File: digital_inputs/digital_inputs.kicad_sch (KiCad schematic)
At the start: 147 parts, among them J1 6437288-2, J10 Conn_01x01, J11 Conn_01x01, J12 Conn_01x01, J13 Conn_01x01, J14 Conn_01x01, J15 Conn_01x01, J16 Conn_01x01, J17 Conn_01x01, J18 Conn_02x05_Odd_Even, J19 6437288-3, J2 Conn_02x07_Odd_Even, J20 Conn_02x24_Odd_Even, J21 Conn_02x08_Odd_Even, J22 Conn_02x15_Odd_Even, J23 Conn_02x10_Odd_Even, J24 Conn_02x17_Odd_Even, J25 Conn_02x10_Odd_Even, J26 Conn_02x06_Odd_Even, J27 Conn_02x16_Odd_Even, J28 Conn_02x04_Odd_Even, J3 Conn_01x08, J4 Conn_01x01, J5 Conn_01x02, J6 Conn_01x04, J7 Conn_01x04, J8 Conn_01x04, J9 Conn_01x04, Q1 AO3400A, Q2 AO3400A, Q3 AO3400A, Q4 AO3400A, Q5 AO3400A, Q6 AO3400A, Q7 AO3400A, Q8 AO3400A, U1 OPA4192IPW, U10 ULN2003A, U12 TJA1051T-3, U2 CD4067BM96, U3 CD4067BM96, U4 CD4067BM96, U5 CD4067BM96, U6 CD4067BM96, U7 CD4067BM96, U8 TC4427, U9 TC4427

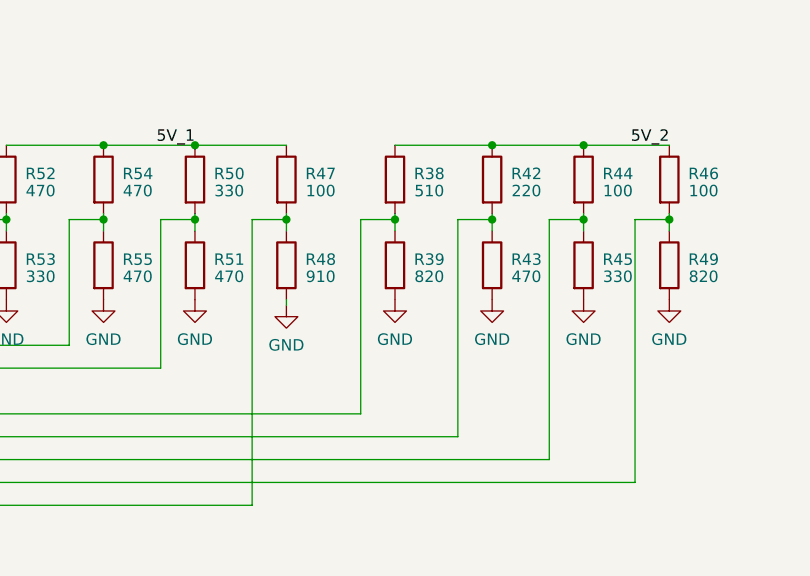
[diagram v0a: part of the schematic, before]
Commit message: check
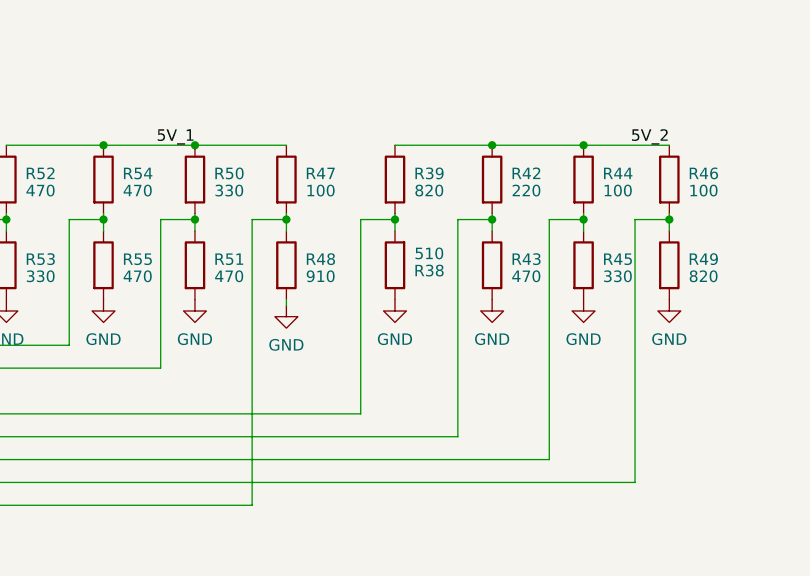
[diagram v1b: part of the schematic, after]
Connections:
- net 5V_2: now also R39.1; no longer R38.1
- net GND: now also R38.1; no longer R39.2
- net REF12: now also R39.2; no longer R39.1
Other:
- moved on the sheet: R38, R39
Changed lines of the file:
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@@
     (stroke (width 0) (type default))
   )
-  (wire (pts (xy 127 356.87) (xy 127 335.28))
+  (wire (pts (xy 127 335.28) (xy 127 356.87))
     (stroke (width 0) (type default))
   )
@@
     )
   )
-  (symbol (lib_id "Device:R") (at 130.81 340.36 0) (unit 1)
-    (in_bom yes) (on_board yes) (dnp no)
-    (property "Reference" "R39" (at 134.62 339.725 0)
-      (effects (font (size 1.27 1.27)))
-    )
-    (property "Value" "820" (at 134.62 341.63 0)
-      (effects (font (size 1.27 1.27)))
-    )
-    (property "Footprint" "Resistor_SMD:R_0603_1608Metric" (at 129.032 340.36 90)
-      (effects (font (size 1.27 1.27)) hide)
-    )
-    (property "Datasheet" "~" (at 130.81 340.36 0)
-      (effects (font (size 1.27 1.27)) hide)
-    )
-    (property "LCSC" "C23253" (at 130.81 340.36 0)
+  (symbol (lib_id "Device:R") (at 130.81 330.835 0) (unit 1)
+    (in_bom yes) (on_board yes) (dnp no)
+    (property "Reference" "R39" (at 134.62 330.2 0)
+      (effects (font (size 1.27 1.27)))
+    )
+    (property "Value" "820" (at 134.62 332.105 0)
+      (effects (font (size 1.27 1.27)))
+    )
+    (property "Footprint" "Resistor_SMD:R_0603_1608Metric" (at 129.032 330.835 90)
+      (effects (font (size 1.27 1.27)) hide)
+    )
+    (property "Datasheet" "~" (at 130.81 330.835 0)
+      (effects (font (size 1.27 1.27)) hide)
+    )
+    (property "LCSC" "C23253" (at 130.81 330.835 0)
       (effects (font (size 1.27 1.27)) hide)
     )
@@
     )
   )
-  (symbol (lib_id "Device:R") (at 130.81 330.835 0) (unit 1)
-    (in_bom yes) (on_board yes) (dnp no)
-    (property "Reference" "R38" (at 134.62 330.2 0)
-      (effects (font (size 1.27 1.27)))
-    )
-    (property "Value" "510" (at 134.62 332.105 0)
-      (effects (font (size 1.27 1.27)))
-    )
-    (property "Footprint" "Resistor_SMD:R_0603_1608Metric" (at 129.032 330.835 90)
-      (effects (font (size 1.27 1.27)) hide)
-    )
-    (property "Datasheet" "~" (at 130.81 330.835 0)
-      (effects (font (size 1.27 1.27)) hide)
-    )
-    (property "LCSC" "C23193" (at 130.81 330.835 0)
-      (effects (font (size 1.27 1.27)) hide)
-    )
+  (symbol (lib_id "Device:R") (at 130.81 340.36 180) (unit 1)
+    (in_bom yes) (on_board yes) (dnp no)
+    (property "Reference" "R38" (at 134.62 340.995 0)
+      (effects (font (size 1.27 1.27)))
+    )
+    (property "Value" "510" (at 134.62 339.09 0)
+      (effects (font (size 1.27 1.27)))
+    )
+    (property "Footprint" "Resistor_SMD:R_0603_1608Metric" (at 132.588 340.36 90)
+      (effects (font (size 1.27 1.27)) hide)
+    )
+    (property "Datasheet" "~" (at 130.81 340.36 0)
+      (effects (font (size 1.27 1.27)) hide)
+    )
+    (property "LCSC" "C23193" (at 130.81 340.36 0)
+      (effects (font (size 1.27 1.27)) hide)
+    )
